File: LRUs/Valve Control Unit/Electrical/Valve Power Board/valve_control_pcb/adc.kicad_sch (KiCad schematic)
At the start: 66 parts, among them U10 ADS124S08IPBSR

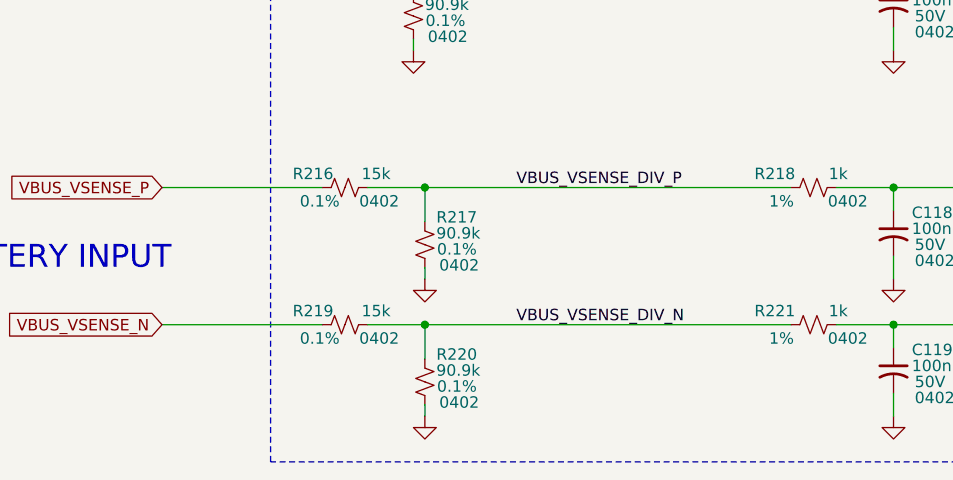
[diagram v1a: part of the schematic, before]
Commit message: Major changes
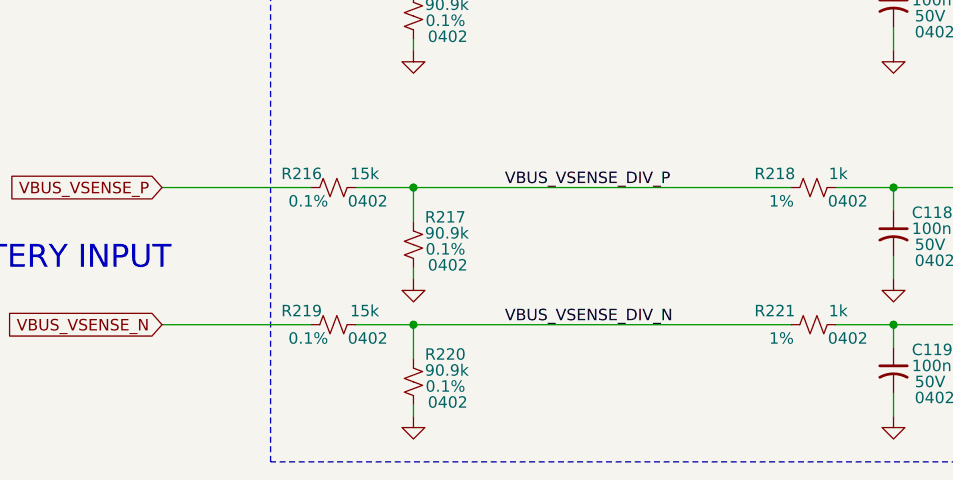
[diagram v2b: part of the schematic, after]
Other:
- moved on the sheet: R216, R217, R219, R220
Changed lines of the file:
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@@
 	(title_block
 		(title "ADC")
-		(date "2026-10-07")
+		(date "2026-10-08")
 		(rev "A")
 	)
@@
 	)
 	(junction
-		(at 100.33 257.81)
+		(at 99.06 257.81)
 		(diameter 0)
 		(color 0 0 0 0)
@@
 	)
 	(junction
-		(at 100.33 242.57)
+		(at 99.06 242.57)
 		(diameter 0)
 		(color 0 0 0 0)
@@
 	(wire
 		(pts
-			(xy 71.12 242.57) (xy 88.9 242.57)
+			(xy 71.12 242.57) (xy 87.63 242.57)
 		)
 		(stroke
@@
 	(wire
 		(pts
-			(xy 100.33 257.81) (xy 140.97 257.81)
+			(xy 99.06 257.81) (xy 140.97 257.81)
 		)
 		(stroke
@@
 	(wire
 		(pts
-			(xy 100.33 251.46) (xy 100.33 252.73)
+			(xy 99.06 251.46) (xy 99.06 252.73)
 		)
 		(stroke
@@
 	(wire
 		(pts
-			(xy 100.33 266.7) (xy 100.33 267.97)
+			(xy 99.06 266.7) (xy 99.06 267.97)
 		)
 		(stroke
@@
 	(wire
 		(pts
-			(xy 100.33 261.62) (xy 100.33 257.81)
+			(xy 99.06 261.62) (xy 99.06 257.81)
 		)
 		(stroke
@@
 	(wire
 		(pts
-			(xy 71.12 257.81) (xy 88.9 257.81)
+			(xy 71.12 257.81) (xy 87.63 257.81)
 		)
 		(stroke
@@
 	(wire
 		(pts
-			(xy 93.98 257.81) (xy 100.33 257.81)
+			(xy 92.71 257.81) (xy 99.06 257.81)
 		)
 		(stroke
@@
 	(wire
 		(pts
-			(xy 100.33 246.38) (xy 100.33 242.57)
+			(xy 99.06 246.38) (xy 99.06 242.57)
 		)
 		(stroke
@@
 	(wire
 		(pts
-			(xy 100.33 242.57) (xy 140.97 242.57)
+			(xy 99.06 242.57) (xy 140.97 242.57)
 		)
 		(stroke
@@
 	(wire
 		(pts
-			(xy 93.98 242.57) (xy 100.33 242.57)
+			(xy 92.71 242.57) (xy 99.06 242.57)
 		)
 		(stroke
@@
 	)
 	(label "VBUS_VSENSE_DIV_P"
-		(at 110.49 242.57 0)
+		(at 109.22 242.57 0)
 		(effects
 			(font
@@
 	)
 	(label "VBUS_VSENSE_DIV_N"
-		(at 110.49 257.81 0)
+		(at 109.22 257.81 0)
 		(effects
 			(font
@@
 	(symbol
 		(lib_id "Device:R_Small_US")
-		(at 100.33 264.16 180)
+		(at 99.06 264.16 180)
 		(unit 1)
 		(body_style 1)
@@
 		(dnp no)
 		(property "Reference" "R220"
-			(at 101.6 261.112 0)
+			(at 100.33 261.112 0)
 			(show_name no)
 			(do_not_autoplace no)
@@
 		)
 		(property "Value" "90.9k"
-			(at 101.6 262.89 0)
+			(at 100.33 262.89 0)
 			(show_name no)
 			(do_not_autoplace no)
@@
 		)
 		(property "Footprint" "valve_pcb_footprints:R_0402_1005Metric_GSE"
-			(at 100.33 264.16 0)
+			(at 99.06 264.16 0)
 			(hide yes)
 			(show_name no)
@@
 		)
 		(property "Datasheet" ""
-			(at 100.33 264.16 0)
+			(at 99.06 264.16 0)
 			(hide yes)
 			(show_name no)
@@
 		)
 		(property "Description" "90.9k 0.1% 0402 Resistor"
-			(at 100.33 264.16 0)
+			(at 99.06 264.16 0)
 			(hide yes)
 			(show_name no)
@@
 		)
 		(property "Tolerance" "0.1%"
-			(at 103.886 264.668 0)
+			(at 102.616 264.668 0)
 			(show_name no)
 			(do_not_autoplace no)
@@
 		)
 		(property "JLCPCB Part #" "C852949"
-			(at 100.33 264.16 0)
+			(at 99.06 264.16 0)
 			(hide yes)
 			(show_name no)
@@
 		)
 		(property "Footprint_Size" "0402"
-			(at 104.14 266.446 0)
+			(at 102.87 266.446 0)
 			(show_name no)
 			(do_not_autoplace no)
@@
 	(symbol
 		(lib_id "power:GND")
-		(at 100.33 267.97 0)
+		(at 99.06 267.97 0)
 		(mirror y)
 		(unit 1)
@@
 		(fields_autoplaced yes)
 		(property "Reference" "#PWR0315"
-			(at 100.33 274.32 0)
+			(at 99.06 274.32 0)
 			(hide yes)
 			(show_name no)
@@
 		)
 		(property "Value" "GND"
-			(at 100.33 273.05 0)
+			(at 99.06 273.05 0)
 			(hide yes)
 			(show_name no)
@@
 		)
 		(property "Footprint" ""
-			(at 100.33 267.97 0)
+			(at 99.06 267.97 0)
 			(hide yes)
 			(show_name no)
@@
 		)
 		(property "Datasheet" ""
-			(at 100.33 267.97 0)
+			(at 99.06 267.97 0)
 			(hide yes)
 			(show_name no)
@@
 		)
 		(property "Description" "Power symbol creates a global label with name \"GND\" , ground"
-			(at 100.33 267.97 0)
+			(at 99.06 267.97 0)
 			(hide yes)
 			(show_name no)
@@
 	(symbol
 		(lib_id "Device:R_Small_US")
-		(at 91.44 257.81 270)
+		(at 90.17 257.81 270)
 		(unit 1)
 		(body_style 1)
@@
 		(dnp no)
 		(property "Reference" "R219"
-			(at 90.17 256.286 90)
+			(at 88.9 256.286 90)
 			(show_name no)
 			(do_not_autoplace no)
@@
 		)
 		(property "Value" "15k"
-			(at 96.52 256.286 90)
+			(at 95.25 256.286 90)
 			(show_name no)
 			(do_not_autoplace no)
@@
 		)
 		(property "Footprint" "valve_pcb_footprints:R_0402_1005Metric_GSE"
-			(at 91.44 257.81 0)
+			(at 90.17 257.81 0)
 			(hide yes)
 			(show_name no)
@@
 		)
 		(property "Datasheet" ""
-			(at 91.44 257.81 0)
+			(at 90.17 257.81 0)
 			(hide yes)
 			(show_name no)
@@
 		)
 		(property "Description" "10k 0.1% 0402 Resistor"
-			(at 91.44 257.81 0)
+			(at 90.17 257.81 0)
 			(hide yes)
 			(show_name no)
@@
 		)
 		(property "Tolerance" "0.1%"
-			(at 88.646 259.334 90)
+			(at 87.376 259.334 90)
 			(show_name no)
 			(do_not_autoplace no)
@@
 		)
 		(property "JLCPCB Part #" "C190095"
-			(at 91.44 257.81 0)
+			(at 90.17 257.81 0)
 			(hide yes)
 			(show_name no)
@@
 		)
 		(property "Footprint_Size" "0402"
-			(at 95.25 259.334 90)
+			(at 93.98 259.334 90)
 			(show_name no)
 			(do_not_autoplace no)
@@
 	(symbol
 		(lib_id "Device:R_Small_US")
-		(at 91.44 242.57 270)
+		(at 90.17 242.57 270)
 		(unit 1)
 		(body_style 1)
@@
 		(dnp no)
 		(property "Reference" "R216"
-			(at 90.17 241.046 90)
+			(at 88.9 241.046 90)
 			(show_name no)
 			(do_not_autoplace no)
@@
 		)
 		(property "Value" "15k"
-			(at 96.52 241.046 90)
+			(at 95.25 241.046 90)
 			(show_name no)
 			(do_not_autoplace no)
@@
 		)
 		(property "Footprint" "valve_pcb_footprints:R_0402_1005Metric_GSE"
-			(at 91.44 242.57 0)
+			(at 90.17 242.57 0)
 			(hide yes)
 			(show_name no)
@@
 		)
 		(property "Datasheet" ""
-			(at 91.44 242.57 0)
+			(at 90.17 242.57 0)
 			(hide yes)
 			(show_name no)
@@
 		)
 		(property "Description" "10k 0.1% 0402 Resistor"
-			(at 91.44 242.57 0)
+			(at 90.17 242.57 0)
 			(hide yes)
 			(show_name no)
@@
 		)
 		(property "Tolerance" "0.1%"
-			(at 88.646 244.094 90)
+			(at 87.376 244.094 90)
 			(show_name no)
 			(do_not_autoplace no)
@@
 		)
 		(property "JLCPCB Part #" "C190095"
-			(at 91.44 242.57 0)
+			(at 90.17 242.57 0)
 			(hide yes)
 			(show_name no)
@@
 		)
 		(property "Footprint_Size" "0402"
-			(at 95.25 244.094 90)
+			(at 93.98 244.094 90)
 			(show_name no)
 			(do_not_autoplace no)
@@
 	(symbol
 		(lib_id "Device:R_Small_US")
-		(at 100.33 248.92 180)
+		(at 99.06 248.92 180)
 		(unit 1)
 		(body_style 1)
@@
 		(dnp no)
 		(property "Reference" "R217"
-			(at 101.6 245.872 0)
+			(at 100.33 245.872 0)
 			(show_name no)
 			(do_not_autoplace no)
@@
 		)
 		(property "Value" "90.9k"
-			(at 101.6 247.65 0)
+			(at 100.33 247.65 0)
 			(show_name no)
 			(do_not_autoplace no)
@@
 		)
 		(property "Footprint" "valve_pcb_footprints:R_0402_1005Metric_GSE"
-			(at 100.33 248.92 0)
+			(at 99.06 248.92 0)
 			(hide yes)
 			(show_name no)
@@
 		)
 		(property "Datasheet" ""
-			(at 100.33 248.92 0)
+			(at 99.06 248.92 0)
 			(hide yes)
 			(show_name no)
@@
 		)
 		(property "Description" "90.9k 0.1% 0402 Resistor"
-			(at 100.33 248.92 0)
+			(at 99.06 248.92 0)
 			(hide yes)
 			(show_name no)
@@
 		)
 		(property "Tolerance" "0.1%"
-			(at 103.886 249.428 0)
+			(at 102.616 249.428 0)
 			(show_name no)
 			(do_not_autoplace no)
@@
 		)
 		(property "JLCPCB Part #" "C852949"
-			(at 100.33 248.92 0)
+			(at 99.06 248.92 0)
 			(hide yes)
 			(show_name no)
@@
 		)
 		(property "Footprint_Size" "0402"
-			(at 104.14 251.206 0)
+			(at 102.87 251.206 0)
 			(show_name no)
 			(do_not_autoplace no)
@@
 	(symbol
 		(lib_id "power:GND")
-		(at 100.33 252.73 0)
+		(at 99.06 252.73 0)
 		(mirror y)
 		(unit 1)
@@
 		(fields_autoplaced yes)
 		(property "Reference" "#PWR0314"
-			(at 100.33 259.08 0)
+			(at 99.06 259.08 0)
 			(hide yes)
 			(show_name no)
@@
 		)
 		(property "Value" "GND"
-			(at 100.33 257.81 0)
+			(at 99.06 257.81 0)
 			(hide yes)
 			(show_name no)
@@
 		)
 		(property "Footprint" ""
-			(at 100.33 252.73 0)
+			(at 99.06 252.73 0)
 			(hide yes)
 			(show_name no)
@@
 		)
 		(property "Datasheet" ""
-			(at 100.33 252.73 0)
+			(at 99.06 252.73 0)
 			(hide yes)
 			(show_name no)
@@
 		)
 		(property "Description" "Power symbol creates a global label with name \"GND\" , ground"
-			(at 100.33 252.73 0)
+			(at 99.06 252.73 0)
 			(hide yes)
 			(show_name no)
